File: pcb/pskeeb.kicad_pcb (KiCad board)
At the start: 2 copper layers, 136.5 x 99.5 mm, 29 parts, among them K11 KEYSW, K12 KEYSW, K13 KEYSW, K14 KEYSW, K15 KEYSW, K21 KEYSW, K22 KEYSW, K23 KEYSW, K24 KEYSW, K25 KEYSW, K31 KEYSW, K32 KEYSW, K33 KEYSW, K34 KEYSW, K35 KEYSW, K41 KEYSW, K42 KEYSW, K43 KEYSW, U1 YAAJ_WeAct_BlackPill_Part_Like, U2 PS/2_Trackpoint, U3 JoyStick

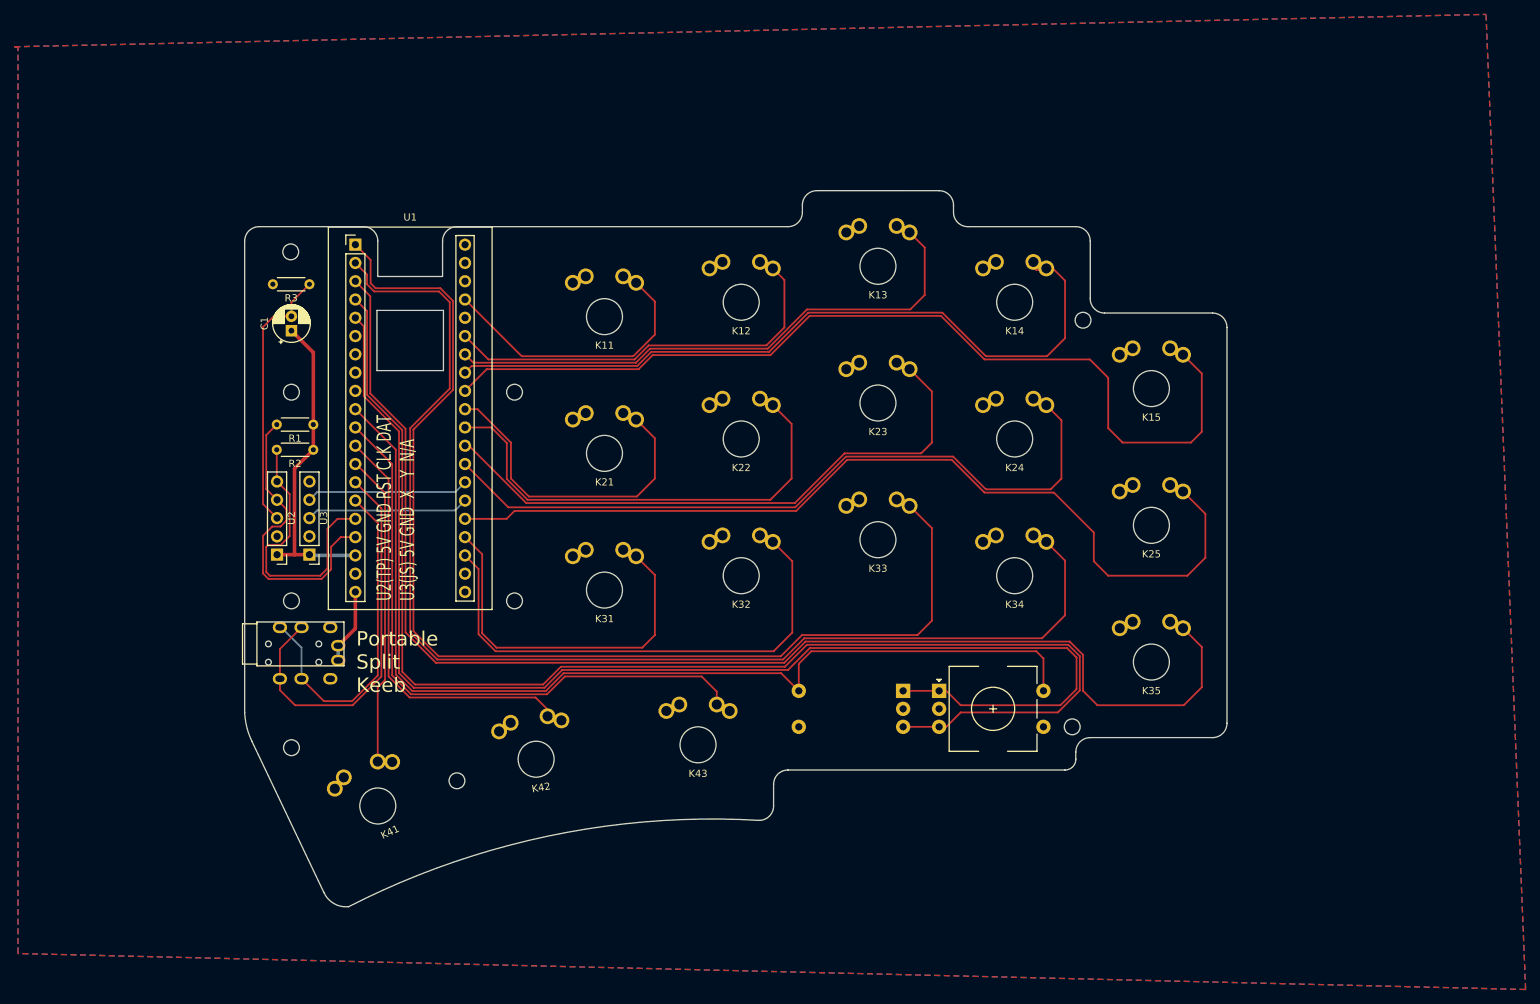
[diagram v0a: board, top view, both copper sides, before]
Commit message: feat: first production
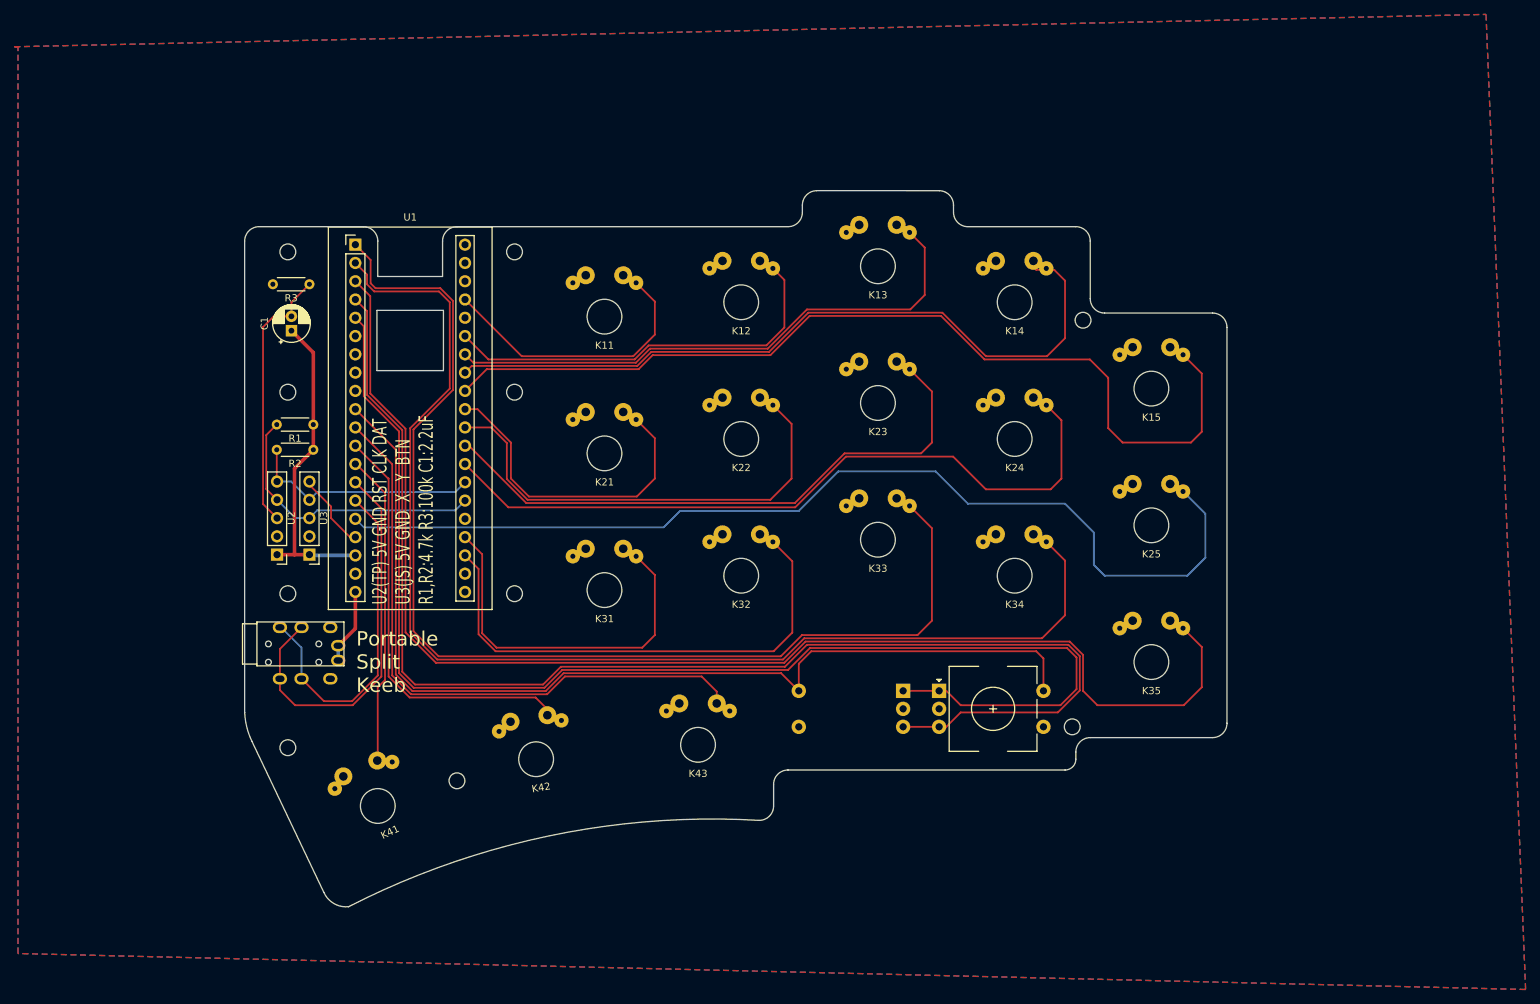
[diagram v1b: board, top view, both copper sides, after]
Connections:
- R1 pad 2: /ps/2_clk -> /joystick_x
- R2 pad 2: /ps/2_dat -> /joystick_y
- U1 pad 16: /ps/2_dat -> /k25
- U1 pad 17: /ps/2_clk -> /joystick_btn
- U1 pad 25: /k25 -> unconnected-(U1-Pad25)
- U2 pad 4: /ps/2_clk -> /joystick_x
- U2 pad 5: /ps/2_dat -> /joystick_y
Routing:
- net /ps/2_clk: track 41.9 -> 0.00 mm
- net /ps/2_dat: track 39.2 -> 0.00 mm
- net /joystick_x: track 22.6 -> 39.9 mm
- net /k25: track 126.8 -> 142.0 mm
- net /joystick_btn: track 0.00 -> 10.8 mm
- net /joystick_y: track 22.6 -> 32.6 mm
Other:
- outline, holes or cut-outs redrawn
- board text added: "U2(TP) 5V GND RST CLK DAT U3(JS) 5V GND X Y BTN R1,R2:4.7k R3:100k C1:2.2uF"
- board text removed: "U2(TP) 5V GND RST CLK DAT U3(JS) 5V GND X Y N/A"
